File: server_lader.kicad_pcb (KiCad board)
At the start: 2 copper layers, 100 x 80 mm, 77 parts, among them IC1 ATMEGA168PA-A, IC2 DAC8560, P1 5V_Vbatt, P10 DISPLAY_STECKER, P11 on/off, P12 A_regulation_out, P2 DISPLAY_STECKER, P3 CONN_02X03, P4 I2C, P5 IP+, P6 IP-, P7 UART, P8 CONN_01X01, P9 Drehrad, U1 ACS758, U2 LTV-356T, U3 ADUM3441, U4 RD-0512D, U5 TPS7A4901, U6 OPA188, U7 LM4040, Y1 RESONATEUR

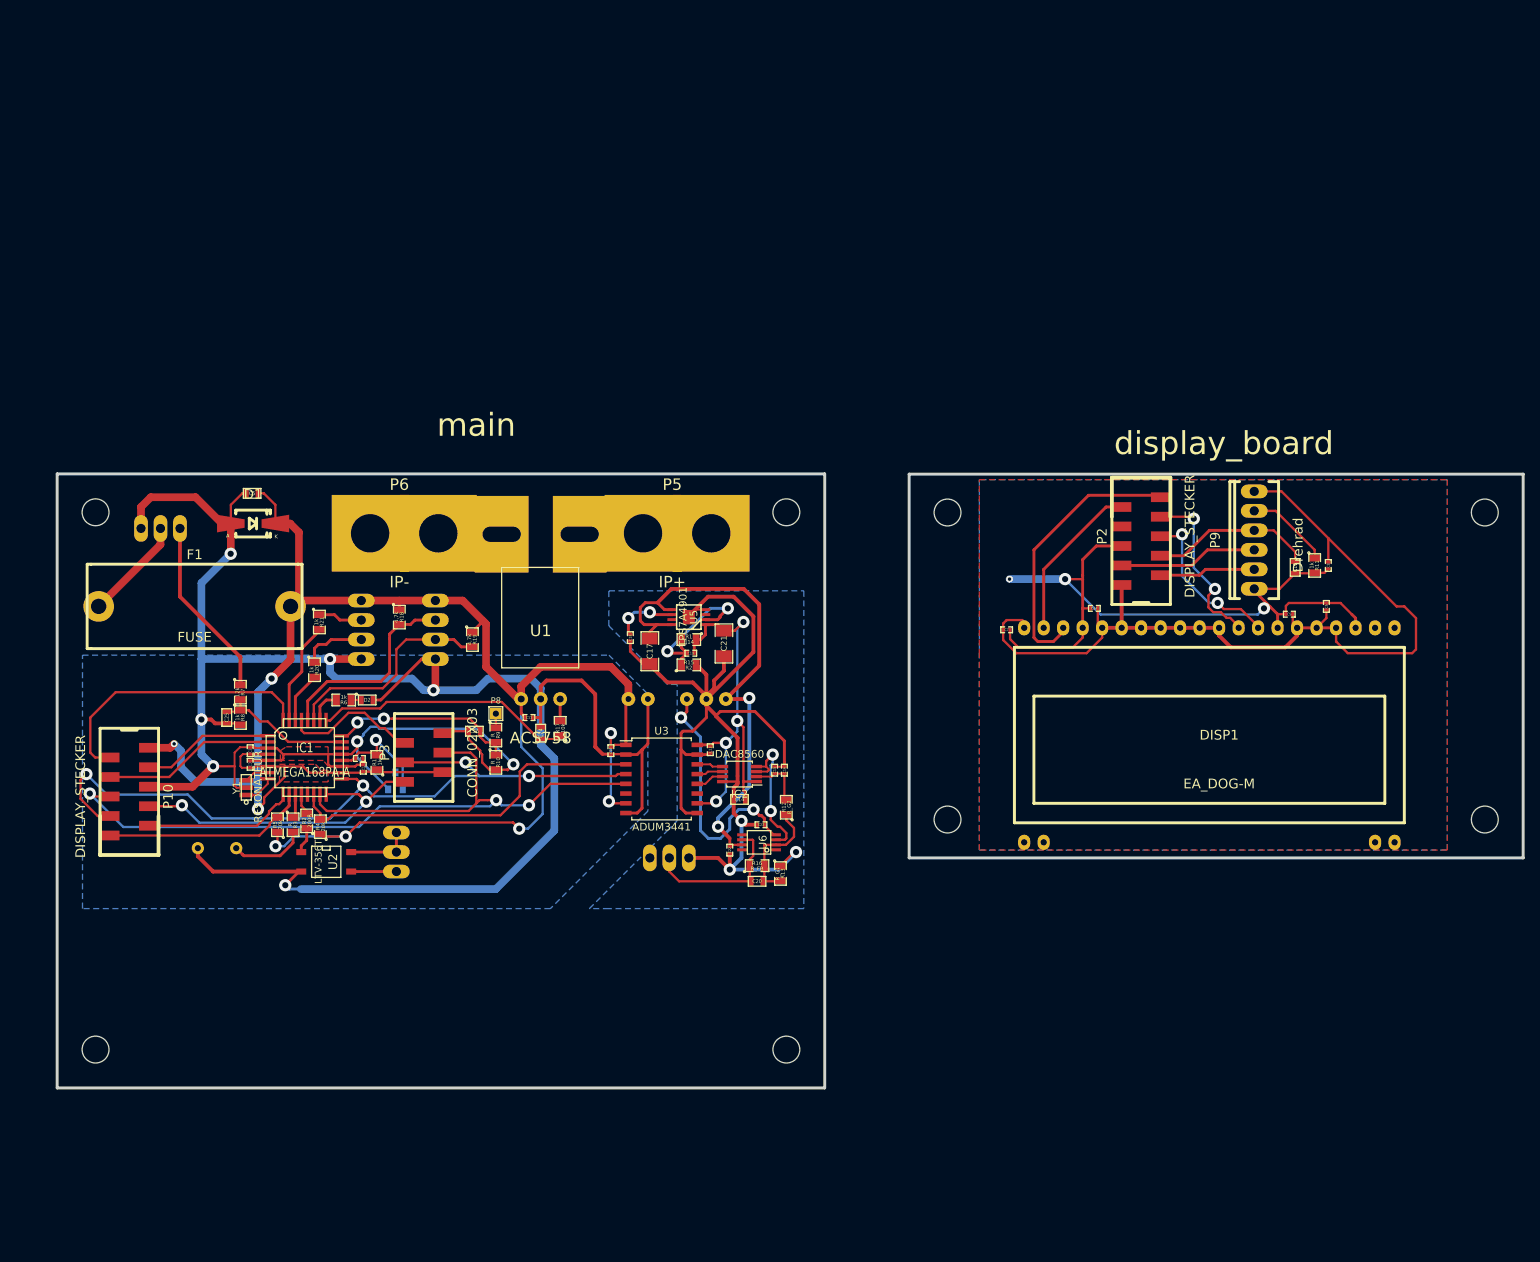
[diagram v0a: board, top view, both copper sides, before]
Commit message: kleine Änderungen
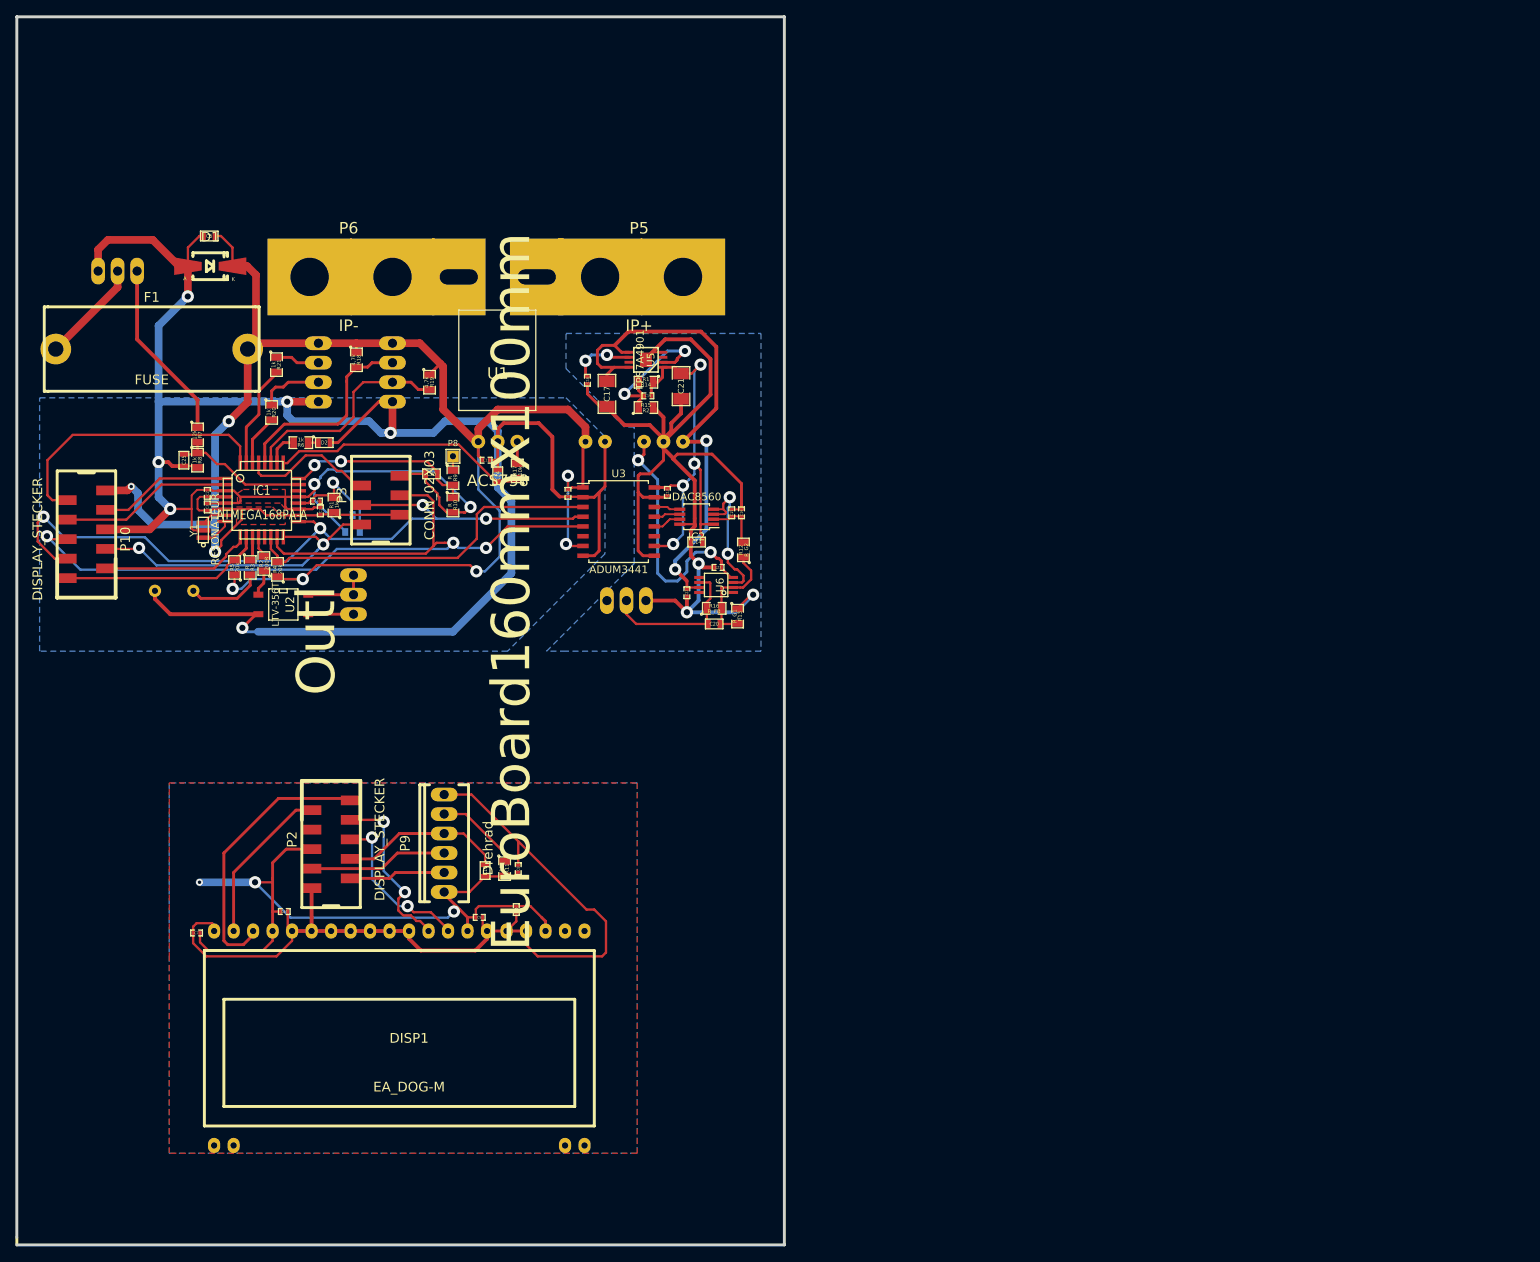
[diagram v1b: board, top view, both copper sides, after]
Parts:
- removed display_board: EuroBoard_viertel_Type-I_80mmX50mm_holes, EuroBoard_Outline:EuroBoard_viertel_Type-I_80mmX50mm_holes
- removed main: EuroBoard_halb_Type-I_100mmX80mm_holes, EuroBoard_Outline:EuroBoard_halb_Type-I_100mmX80mm_holes
- added Outl: EuroBoard160mmX100mm, EuroBoard_Outline:EuroBoard160mmX100mm, F.Cu at (162.6, 173.4)
- moved C10 112.7 mm to (123.6, 124.6)
- moved C9 112.7 mm to (122.8, 130.7)
- moved P2 112.7 mm to (103.5, 120.5)
- moved P9 112.7 mm to (118.2, 121.0)
- moved C27 112.7 mm to (97.4, 129.9)
- moved C6 112.7 mm to (127.6, 129.7)
- moved C7 112.7 mm to (86.0, 132.7)
- moved C8 112.7 mm to (127.9, 124.3)
- moved DISP1 112.7 mm to (113.7, 147.7)
- moved R11 112.7 mm to (126.1, 124.3)
- moved P6 34.0 mm to (105.8, 47.2)
- moved C24 34.0 mm to (125.2, 73.2)
- moved C26 34.0 mm to (116.6, 72.9)
- moved C4 34.0 mm to (101.6, 76.5)
- moved C5 34.0 mm to (87.6, 41.9)
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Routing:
- net Net-(P6-Pad1): track 17.2 -> 19.6 mm
- net Net-(P5-Pad1): track 17.2 -> 19.2 mm
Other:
- board size 100 x 80 mm -> 100 x 160 mm
